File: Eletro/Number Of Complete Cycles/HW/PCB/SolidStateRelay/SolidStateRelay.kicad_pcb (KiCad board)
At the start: 2 copper layers, 62.5 x 27.5 mm, 13 parts, among them J1 KRE_02, Q1 BT138-600, U1 MOC3020M

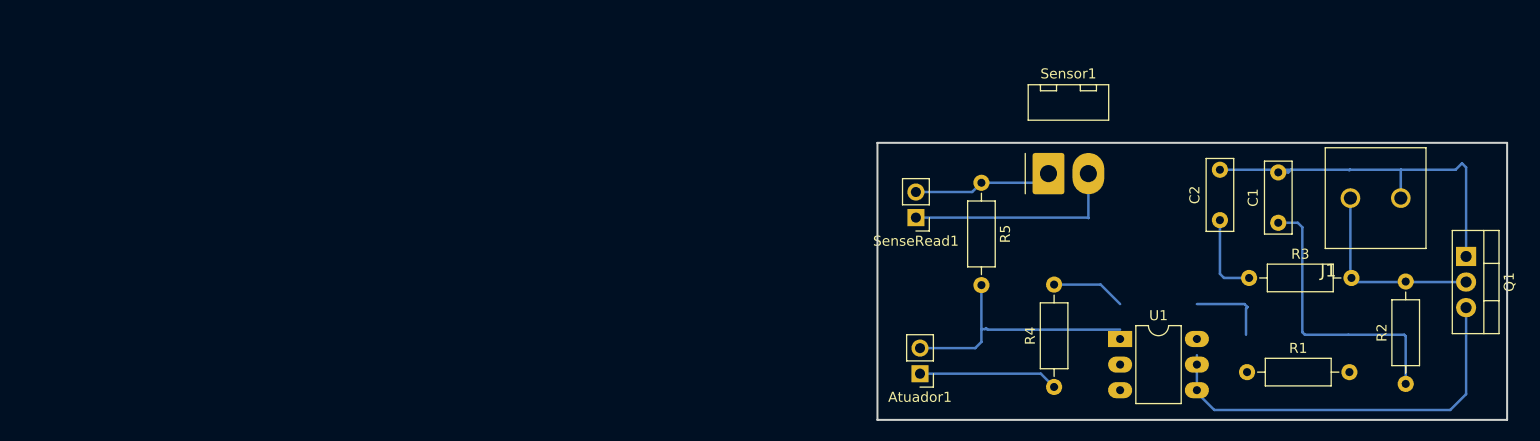
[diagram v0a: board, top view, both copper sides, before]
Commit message: PCB update
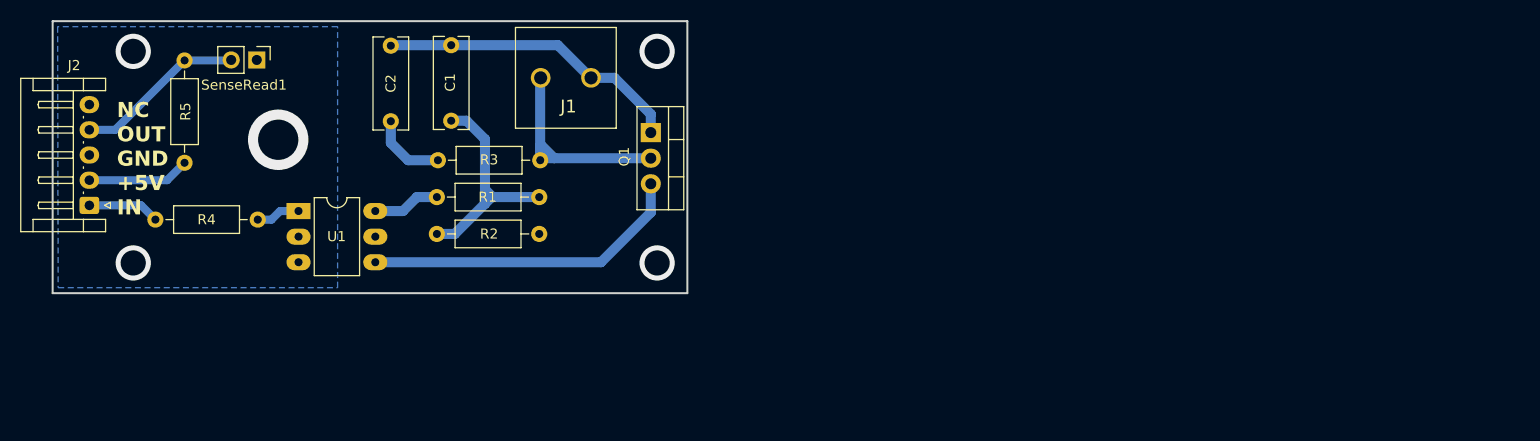
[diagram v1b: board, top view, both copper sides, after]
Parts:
- removed Atuador1: ~, Connector_PinHeader_2.54mm:PinHeader_1x02_P2.54mm_Vertical
- removed Sensor1: ~, Connector_Molex:Molex_KK-396_A-41792-0002_1x02_P3.96mm_Horizontal
- added J2: Conn_01x05_Pin, Connector_JST:JST_EH_S5B-EH_1x05_P2.50mm_Horizontal, F.Cu at (53.6, 68.3)
- C1: value 47n -> 330n; footprint Capacitor_THT:C_Disc_D7.0mm_W2.5mm_P5.00mm -> Capacitor_THT:C_Rect_L9.0mm_W3.3mm_P7.50mm_MKT
- C2: value 10n -> 220n; footprint Capacitor_THT:C_Disc_D7.0mm_W2.5mm_P5.00mm -> Capacitor_THT:C_Rect_L9.0mm_W3.3mm_P7.50mm_MKT
- R1: value 360 -> 330
- R2: value 470 -> 510
- R3: value 39 -> 47
- moved R2 97.3 mm to (88.1, 71.1), turned to 0 degrees
- moved R4 90.7 mm to (60.2, 69.7), turned to 0 degrees
- moved C2 82.9 mm to (83.6, 59.9)
- moved C1 82.7 mm to (89.6, 59.9)
- moved U1 82.5 mm to (74.4, 68.8)
- moved R1 82.3 mm to (88.1, 67.5)
- moved Q1 81.9 mm to (109.4, 61.1)
- moved R3 81.4 mm to (88.2, 63.8)
- moved R5 80.0 mm to (63.1, 53.9)
- moved J1 76.3 mm to (103.4, 55.6), turned to 180 degrees
- moved SenseRead1 67.3 mm to (70.3, 53.8), turned to -90 degrees
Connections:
- J1 pad 1: Net-(Q1-A2) -> Net-(Q1-A1)
- J1 pad 2: Net-(Q1-A1) -> Net-(Q1-A2)
- R5 pad 2: Net-(Atuador1-Pin_2) -> +5V
- SenseRead1 pad 1: Net-(SenseRead1-Pin_1) -> GND
- U1 pad 2: Net-(Atuador1-Pin_2) -> GND
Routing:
- net Net-(Atuador1-Pin_2): track 25.9 -> 0.00 mm
- net Net-(SenseRead1-Pin_1): track 21.5 -> 0.00 mm
- net +5V: track 0.00 -> 10.2 mm
- net Net-(Q1-G): track 40.4 -> 32.2 mm
- net Net-(Q1-A1): track 38.0 -> 30.5 mm
- net Net-(J2-Pin_1): track 13.9 -> 7.14 mm
- net Net-(C1-Pad1): track 28.1 -> 24.2 mm
- net Net-(J2-Pin_4): track 13.9 -> 17.0 mm
- net Net-(R4-Pad2): track 7.35 -> 4.49 mm
- net Net-(Q1-A2): track 19.5 -> 21.3 mm
- net Net-(R1-Pad1): track 7.96 -> 6.69 mm
- net Net-(C2-Pad1): track 8.40 -> 7.48 mm
- net (no net): vias 0 -> 5
- added copper zone on B.Cu, net GND
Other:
- board size 62.5 x 27.5 mm -> 63 x 27 mm
- board text added: "NC OUT GND +5V IN"
